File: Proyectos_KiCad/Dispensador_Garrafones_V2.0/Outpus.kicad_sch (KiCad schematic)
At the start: 42 parts, among them J10 LOAD, J5 LOAD, J6 LOAD, J7 LOAD, J8 LOAD, J9 LOAD, Q1 TIP122, Q2 BT136-800, Q3 BT136-800, Q4 BT136-800, Q5 BT136-800, U3 PC817, U4 MOC3021M, U5 MOC3021M, U6 MOC3021M, U7 MOC3021M

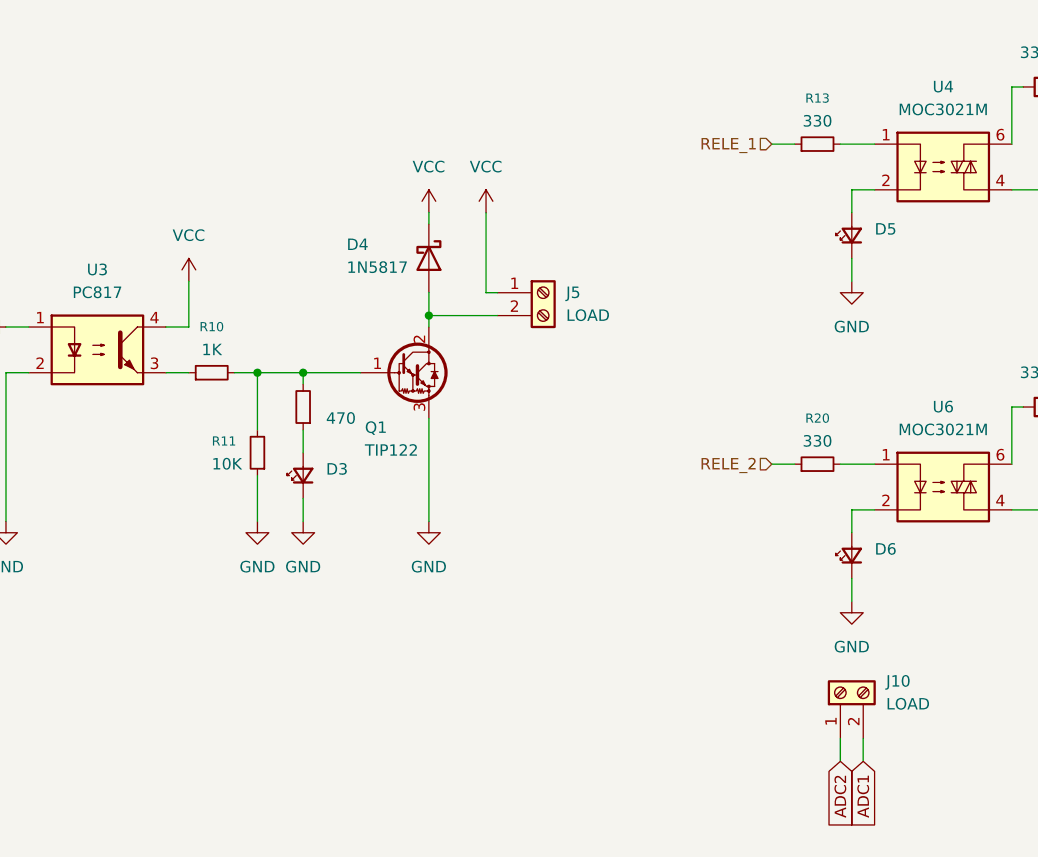
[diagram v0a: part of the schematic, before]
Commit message: Nuevos Proyectos
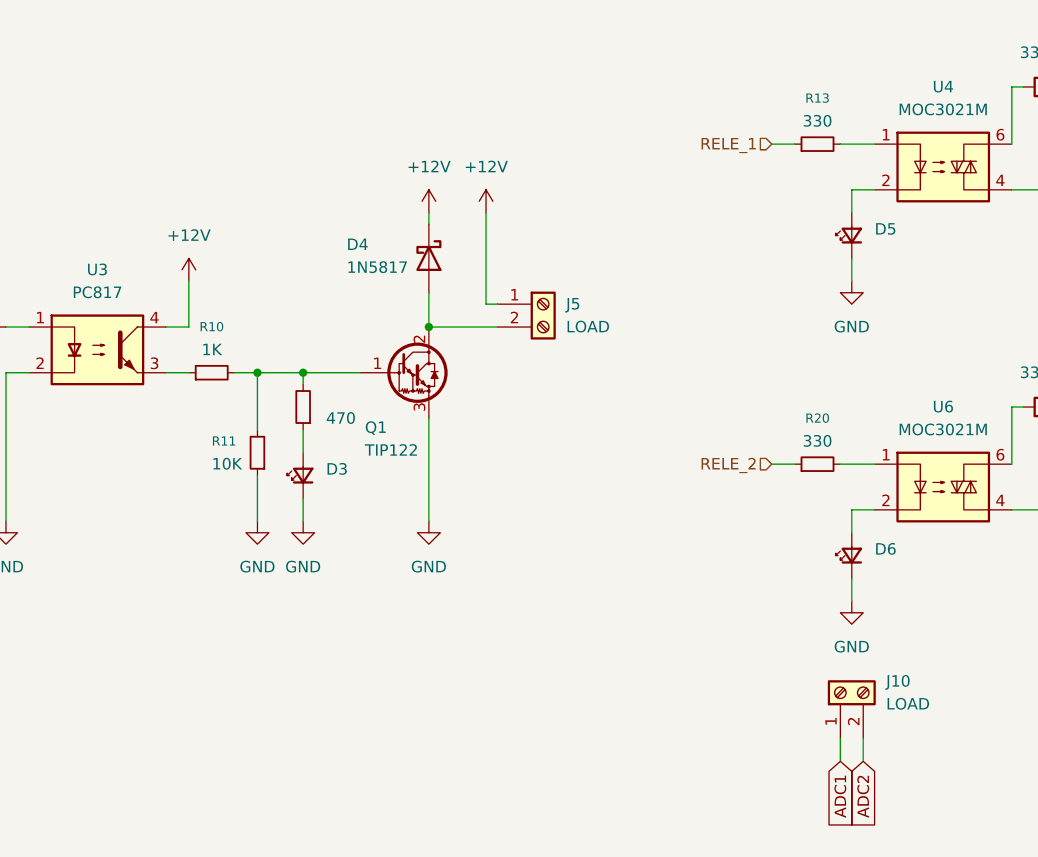
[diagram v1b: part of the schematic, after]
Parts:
- Q1, Q2, Q3, Q4, Q5: footprint Package_TO_SOT_THT:TO-220-3_Vertical -> @EmersonPrez15:TO-220-3_VDC
- R15, R18, R22, R23: footprint PCM_Resistor_THT_AKL:R_Axial_DIN0207_L6.3mm_D2.5mm_P15.24mm_Horizontal -> Resistor_THT:R_Axial_DIN0207_L6.3mm_D2.5mm_P10.16mm_Horizontal
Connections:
- net ADC1: now also J10.1 (Pin_1); no longer J10.2 (Pin_2)
- net ADC2: now also J10.2 (Pin_2); no longer J10.1 (Pin_1)
- net VCC renamed +12V
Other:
- moved on the sheet: J5
